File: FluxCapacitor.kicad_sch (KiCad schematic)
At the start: 37 parts, among them J1 Jack-DC, J2 TM_1, J3 TM_2, J7 TM_1, J8 TM_1, U1 OKI-78SR-5_1.5-W36-C, U2 ESP32_DEVBOARD

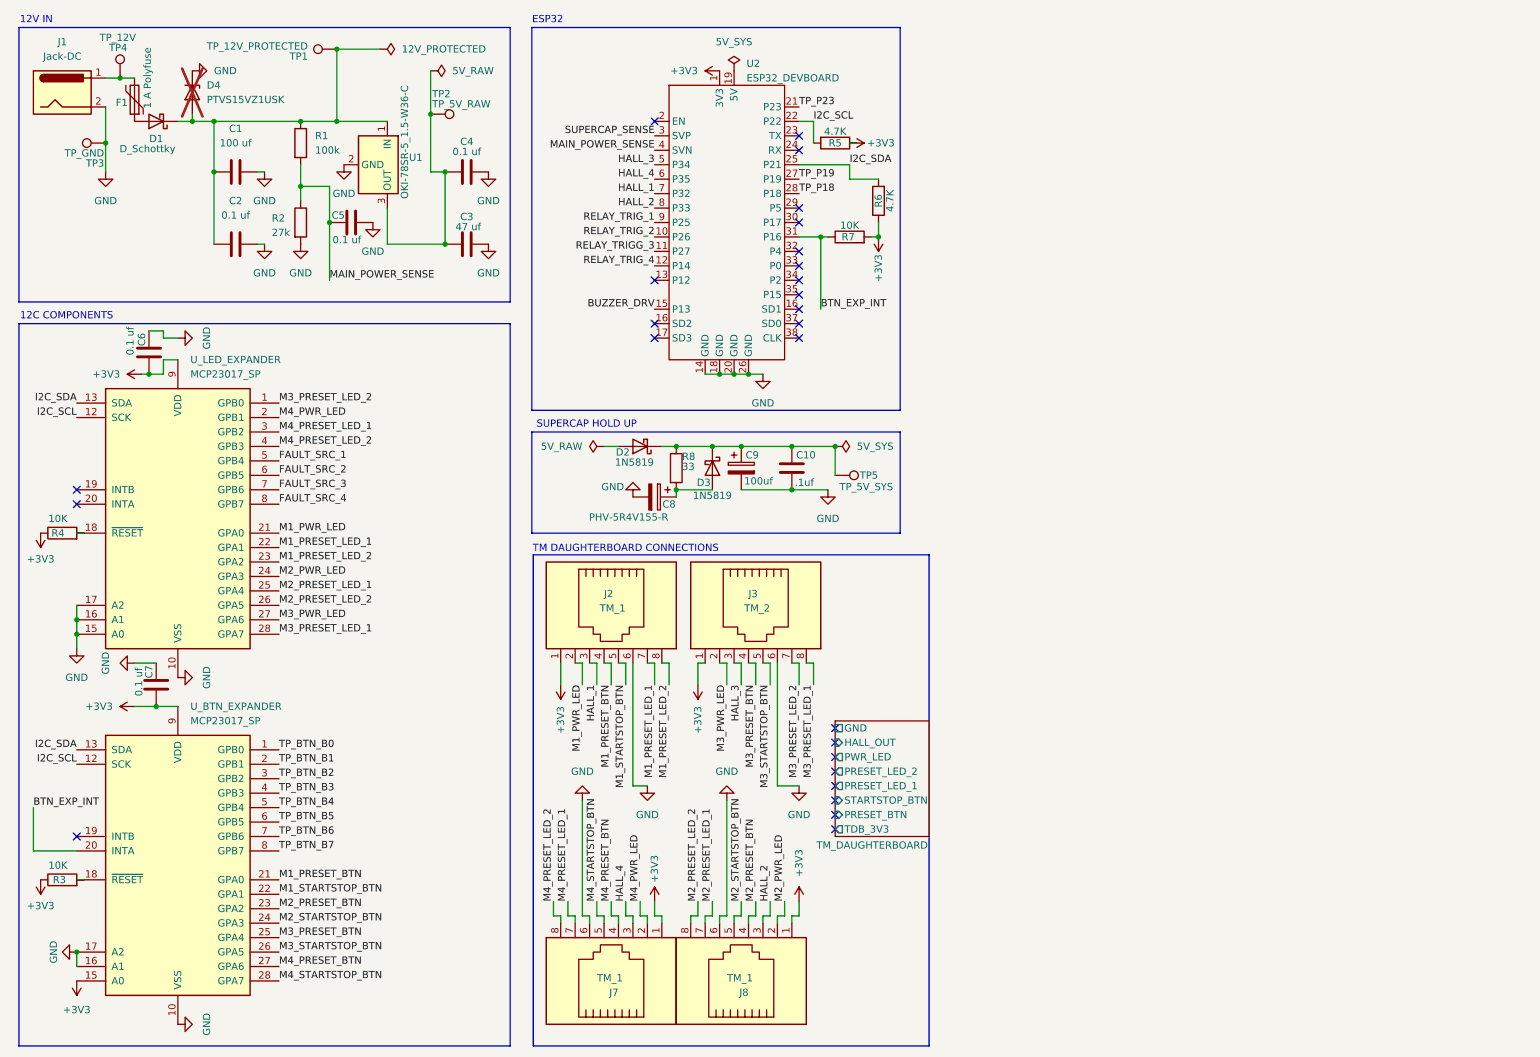
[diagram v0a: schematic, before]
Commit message: Misc save
Started relay-related boards
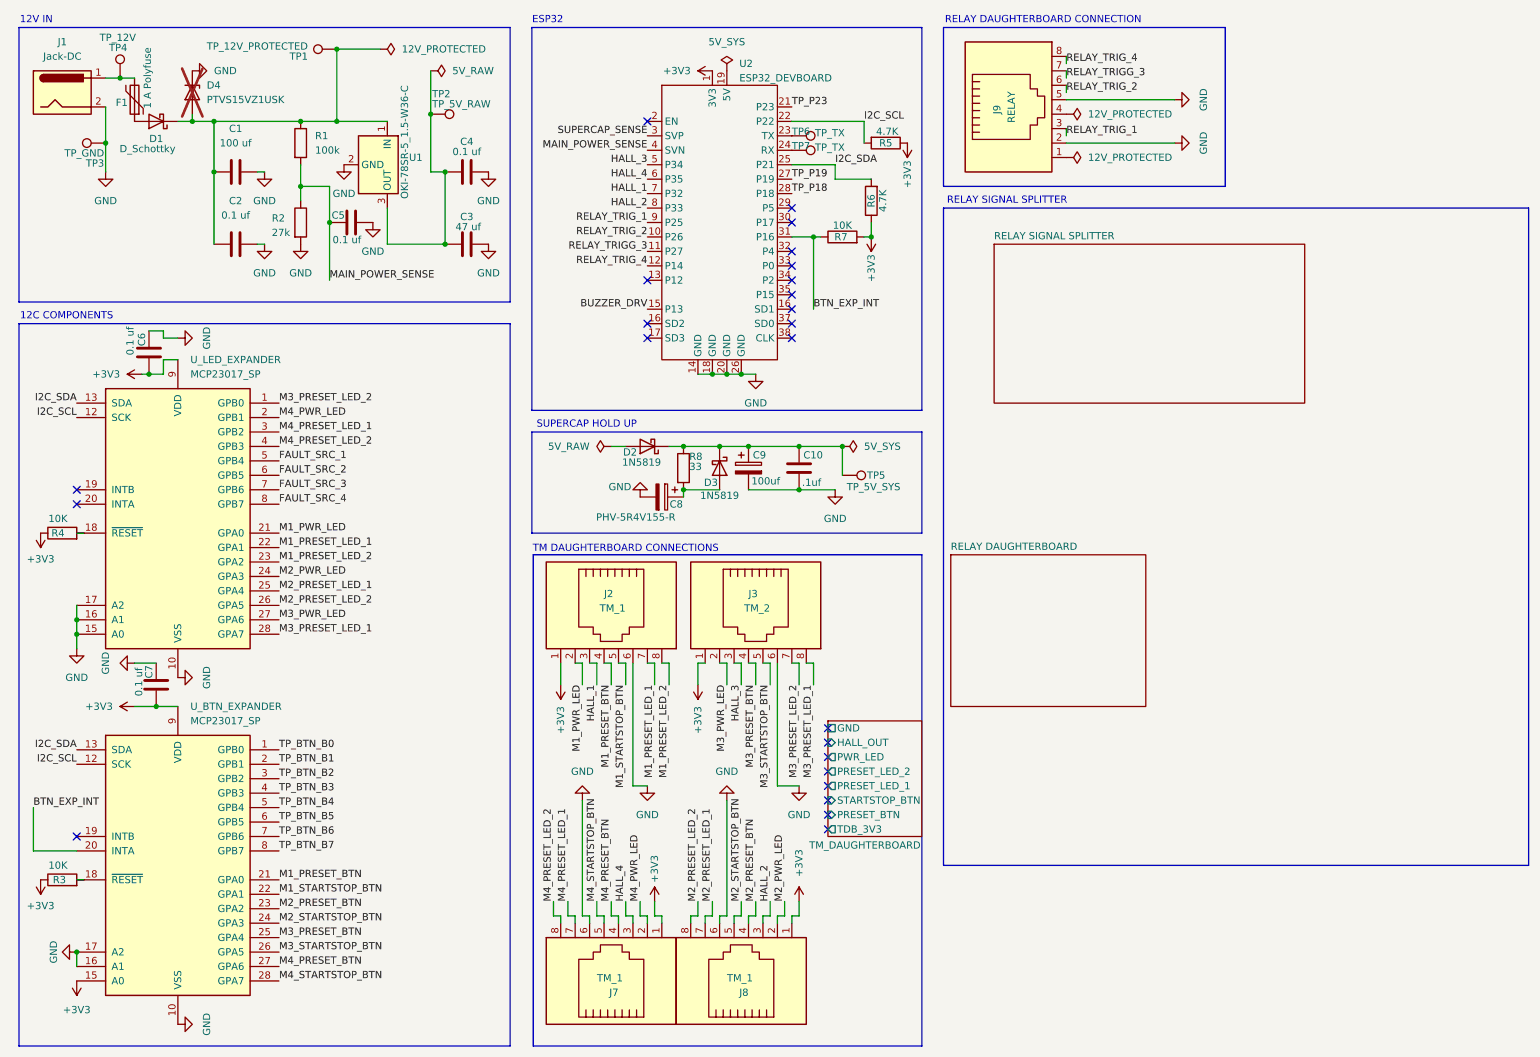
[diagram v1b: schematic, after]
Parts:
- added J9: RELAY, symbol Connector:RJ45
- added TP6, TP7: TP_TX, symbol Connector:TestPoint
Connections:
- net GND: now also J9.2, J9.5
- net RELAY_TRIGG_3: now also J9.7
- net RELAY_TRIG_1: now also J9.3
- net RELAY_TRIG_2: now also J9.6
- net RELAY_TRIG_4: now also J9.8
- net at U2.23 (TX): now also TP6.1
- net at U2.24 (RX): now also TP7.1
- no-connect marks 26 -> 24
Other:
- added sheet RELAY DAUGHTERBOARD (Relay_Daughterboard.kicad_sch)
- added sheet RELAY SIGNAL SPLITTER (RELAY_SIGNAL_SPLITTER.kicad_sch)
- note added: "RELAY DAUGHTERBOARD CONNECTION"
- note added: "RELAY SIGNAL SPLITTER"
- moved on the sheet: C10, C8, C9, D2, D3, R5, R6, R7, R8, TP5, U2
